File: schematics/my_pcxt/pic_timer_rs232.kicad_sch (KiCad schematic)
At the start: 17 parts, among them J3 Conn_02x40_Top_Bottom, J5 DE9_Plug, U14 16550, U15 8253, U23 DTE, U3 PAL20L8, U7 8259A, X1 4.915200MHz

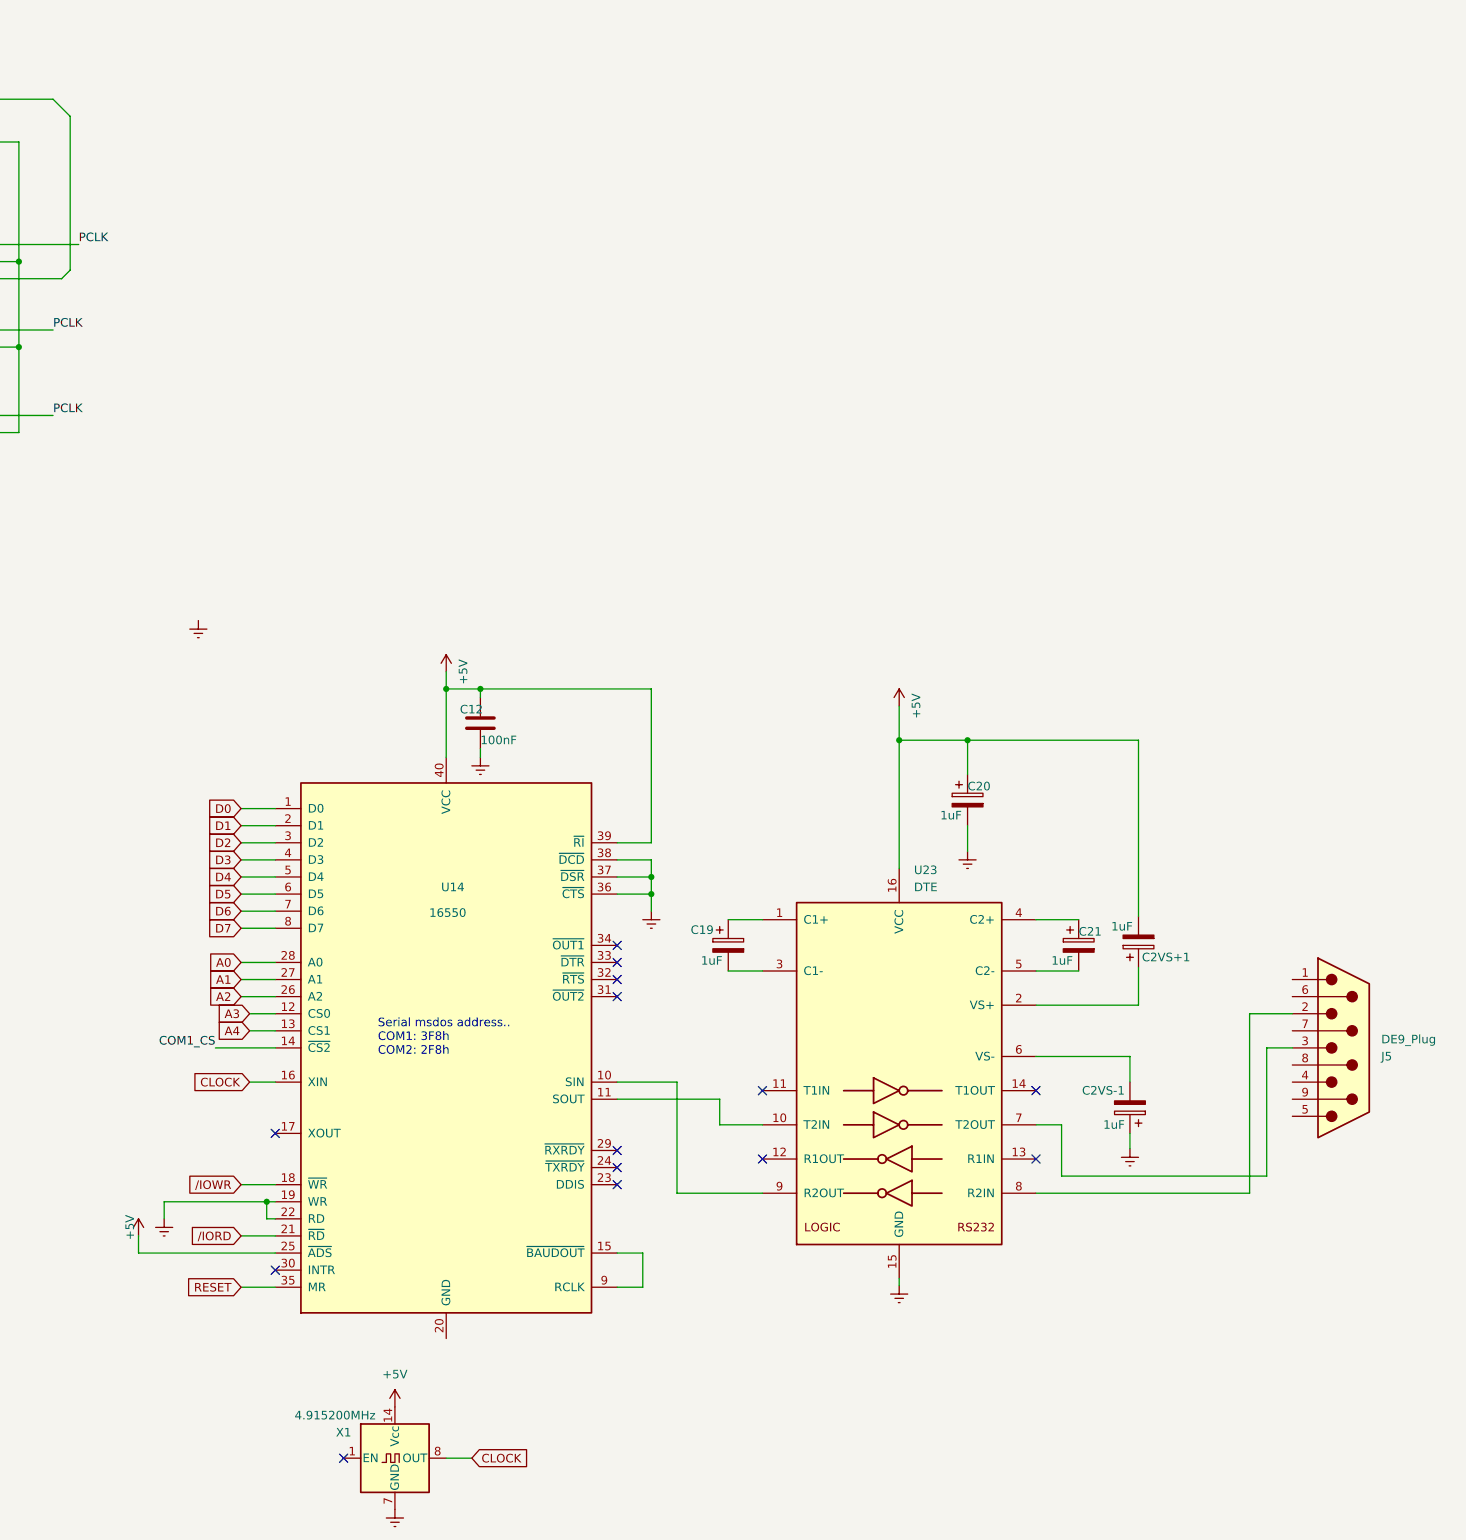
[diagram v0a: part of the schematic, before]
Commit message: Updating schematic
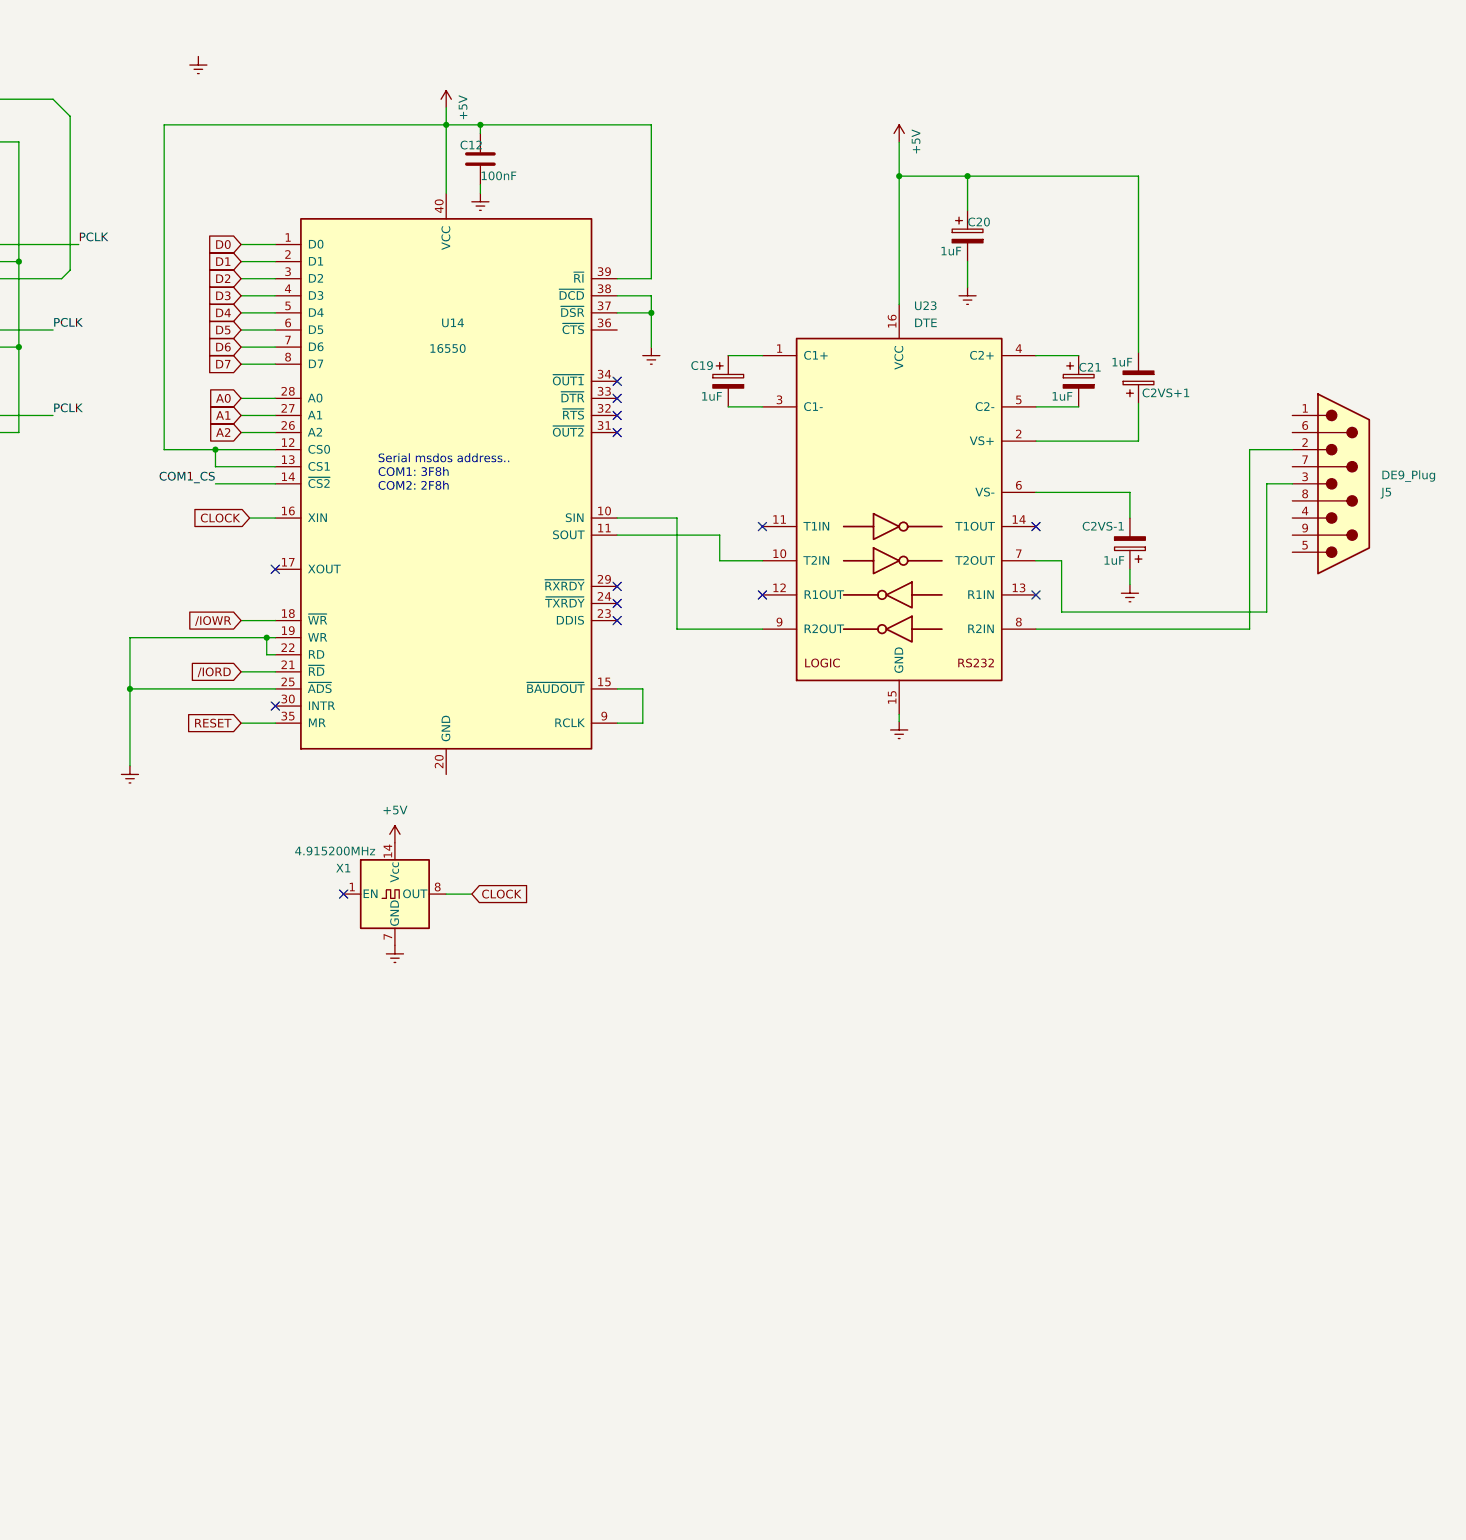
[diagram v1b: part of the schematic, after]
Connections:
- net +5V: now also U14.12 (CS0), U14.13 (CS1); no longer U14.25 (~{ADS})
- net A3: no longer U14.12 (CS0)
- net A4: no longer U14.13 (CS1)
- net GNDREF: now also U14.25 (~{ADS}); no longer U14.36 (~{CTS})
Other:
- moved on the sheet: C12, C19, C20, C21, C2VS+1, C2VS-1, J5, U14, U23, X1
